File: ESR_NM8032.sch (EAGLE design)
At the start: 78 parts, among them J1 0

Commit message: .
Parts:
- C5: device rcl:CPOL-EUE2.5-5 -> rcl:CPOL-EUE2-5
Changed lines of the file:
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@@
 <grid distance="100" unitdist="mil" unit="mil" style="lines" multiple="1" display="yes" altdistance="0.01" altunitdist="inch" altunit="inch"/>
 <layers>
-<layer number="1" name="Top" color="4" fill="1" visible="no" active="no"/>
-<layer number="2" name="Route2" color="1" fill="3" visible="no" active="no"/>
-<layer number="3" name="Route3" color="4" fill="3" visible="no" active="no"/>
-<layer number="4" name="Route4" color="1" fill="4" visible="no" active="no"/>
-<layer number="5" name="Route5" color="4" fill="4" visible="no" active="no"/>
-<layer number="6" name="Route6" color="1" fill="8" visible="no" active="no"/>
-<layer number="7" name="Route7" color="4" fill="8" visible="no" active="no"/>
-<layer number="8" name="Route8" color="1" fill="2" visible="no" active="no"/>
-<layer number="9" name="Route9" color="4" fill="2" visible="no" active="no"/>
-<layer number="10" name="Route10" color="1" fill="7" visible="no" active="no"/>
-<layer number="11" name="Route11" color="4" fill="7" visible="no" active="no"/>
-<layer number="12" name="Route12" color="1" fill="5" visible="no" active="no"/>
-<layer number="13" name="Route13" color="4" fill="5" visible="no" active="no"/>
-<layer number="14" name="Route14" color="1" fill="6" visible="no" active="no"/>
-<layer number="15" name="Route15" color="4" fill="6" visible="no" active="no"/>
-<layer number="16" name="Bottom" color="1" fill="1" visible="no" active="no"/>
-<layer number="17" name="Pads" color="2" fill="1" visible="no" active="no"/>
-<layer number="18" name="Vias" color="2" fill="1" visible="no" active="no"/>
-<layer number="19" name="Unrouted" color="6" fill="1" visible="no" active="no"/>
-<layer number="20" name="Dimension" color="15" fill="1" visible="no" active="no"/>
-<layer number="21" name="tPlace" color="7" fill="1" visible="no" active="no"/>
-<layer number="22" name="bPlace" color="7" fill="1" visible="no" active="no"/>
-<layer number="23" name="tOrigins" color="15" fill="1" visible="no" active="no"/>
-<layer number="24" name="bOrigins" color="15" fill="1" visible="no" active="no"/>
-<layer number="25" name="tNames" color="7" fill="1" visible="no" active="no"/>
-<layer number="26" name="bNames" color="7" fill="1" visible="no" active="no"/>
-<layer number="27" name="tValues" color="7" fill="1" visible="no" active="no"/>
-<layer number="28" name="bValues" color="7" fill="1" visible="no" active="no"/>
+<layer number="1" name="Top" color="4" fill="1" visible="yes" active="no"/>
+<layer number="2" name="Route2" color="1" fill="3" visible="yes" active="no"/>
+<layer number="3" name="Route3" color="4" fill="3" visible="yes" active="no"/>
+<layer number="4" name="Route4" color="1" fill="4" visible="yes" active="no"/>
+<layer number="5" name="Route5" color="4" fill="4" visible="yes" active="no"/>
+<layer number="6" name="Route6" color="1" fill="8" visible="yes" active="no"/>
+<layer number="7" name="Route7" color="4" fill="8" visible="yes" active="no"/>
+<layer number="8" name="Route8" color="1" fill="2" visible="yes" active="no"/>
+<layer number="9" name="Route9" color="4" fill="2" visible="yes" active="no"/>
+<layer number="10" name="Route10" color="1" fill="7" visible="yes" active="no"/>
+<layer number="11" name="Route11" color="4" fill="7" visible="yes" active="no"/>
+<layer number="12" name="Route12" color="1" fill="5" visible="yes" active="no"/>
+<layer number="13" name="Route13" color="4" fill="5" visible="yes" active="no"/>
+<layer number="14" name="Route14" color="1" fill="6" visible="yes" active="no"/>
+<layer number="15" name="Route15" color="4" fill="6" visible="yes" active="no"/>
+<layer number="16" name="Bottom" color="1" fill="1" visible="yes" active="no"/>
+<layer number="17" name="Pads" color="2" fill="1" visible="yes" active="no"/>
+<layer number="18" name="Vias" color="2" fill="1" visible="yes" active="no"/>
+<layer number="19" name="Unrouted" color="6" fill="1" visible="yes" active="no"/>
+<layer number="20" name="Dimension" color="15" fill="1" visible="yes" active="no"/>
+<layer number="21" name="tPlace" color="7" fill="1" visible="yes" active="no"/>
+<layer number="22" name="bPlace" color="7" fill="1" visible="yes" active="no"/>
+<layer number="23" name="tOrigins" color="15" fill="1" visible="yes" active="no"/>
+<layer number="24" name="bOrigins" color="15" fill="1" visible="yes" active="no"/>
+<layer number="25" name="tNames" color="7" fill="1" visible="yes" active="no"/>
+<layer number="26" name="bNames" color="7" fill="1" visible="yes" active="no"/>
+<layer number="27" name="tValues" color="7" fill="1" visible="yes" active="no"/>
+<layer number="28" name="bValues" color="7" fill="1" visible="yes" active="no"/>
 <layer number="29" name="tStop" color="7" fill="3" visible="no" active="no"/>
 <layer number="30" name="bStop" color="7" fill="6" visible="no" active="no"/>
@@
 <layer number="35" name="tGlue" color="7" fill="4" visible="no" active="no"/>
 <layer number="36" name="bGlue" color="7" fill="5" visible="no" active="no"/>
-<layer number="37" name="tTest" color="7" fill="1" visible="no" active="no"/>
-<layer number="38" name="bTest" color="7" fill="1" visible="no" active="no"/>
+<layer number="37" name="tTest" color="7" fill="1" visible="yes" active="no"/>
+<layer number="38" name="bTest" color="7" fill="1" visible="yes" active="no"/>
 <layer number="39" name="tKeepout" color="4" fill="11" visible="no" active="no"/>
 <layer number="40" name="bKeepout" color="1" fill="11" visible="no" active="no"/>
@@
 <layer number="44" name="Drills" color="7" fill="1" visible="no" active="no"/>
 <layer number="45" name="Holes" color="7" fill="1" visible="no" active="no"/>
-<layer number="46" name="Milling" color="3" fill="1" visible="no" active="no"/>
-<layer number="47" name="Measures" color="7" fill="1" visible="no" active="no"/>
-<layer number="48" name="Document" color="7" fill="1" visible="no" active="no"/>
-<layer number="49" name="Reference" color="7" fill="1" visible="no" active="no"/>
-<layer number="50" name="dxf" color="7" fill="1" visible="no" active="no"/>
-<layer number="51" name="tDocu" color="7" fill="1" visible="no" active="no"/>
-<layer number="52" name="bDocu" color="7" fill="1" visible="no" active="no"/>
-<layer number="53" name="tGND_GNDA" color="7" fill="9" visible="no" active="no"/>
-<layer number="54" name="bGND_GNDA" color="1" fill="9" visible="no" active="no"/>
-<layer number="56" name="wert" color="7" fill="1" visible="no" active="no"/>
-<layer number="57" name="tCAD" color="7" fill="1" visible="no" active="no"/>
+<layer number="46" name="Milling" color="3" fill="1" visible="yes" active="no"/>
+<layer number="47" name="Measures" color="7" fill="1" visible="yes" active="no"/>
+<layer number="48" name="Document" color="7" fill="1" visible="yes" active="no"/>
+<layer number="49" name="Reference" color="7" fill="1" visible="yes" active="no"/>
+<layer number="50" name="dxf" color="7" fill="1" visible="yes" active="no"/>
+<layer number="51" name="tDocu" color="7" fill="1" visible="yes" active="no"/>
+<layer number="52" name="bDocu" color="7" fill="1" visible="yes" active="no"/>
+<layer number="53" name="tGND_GNDA" color="7" fill="9" visible="yes" active="no"/>
+<layer number="54" name="bGND_GNDA" color="1" fill="9" visible="yes" active="no"/>
+<layer number="56" name="wert" color="7" fill="1" visible="yes" active="no"/>
+<layer number="57" name="tCAD" color="7" fill="1" visible="yes" active="no"/>
 <layer number="90" name="Modules" color="5" fill="1" visible="yes" active="yes"/>
 <layer number="91" name="Nets" color="2" fill="1" visible="yes" active="yes"/>
@@
 <part name="R8" library="rcl" deviceset="R-EU_" device="R0805" value="10k"/>
 <part name="GND5" library="supply1" deviceset="GND" device=""/>
-<part name="C5" library="rcl" deviceset="CPOL-EU" device="E2.5-5" value="10m"/>
+<part name="C5" library="rcl" deviceset="CPOL-EU" device="E2-5" value="10m"/>
 <part name="R7" library="rcl" deviceset="R-EU_" device="R0805" value="10k"/>
 <part name="C6" library="rcl" deviceset="C-EU" device="075-032X103" value="220n"/>

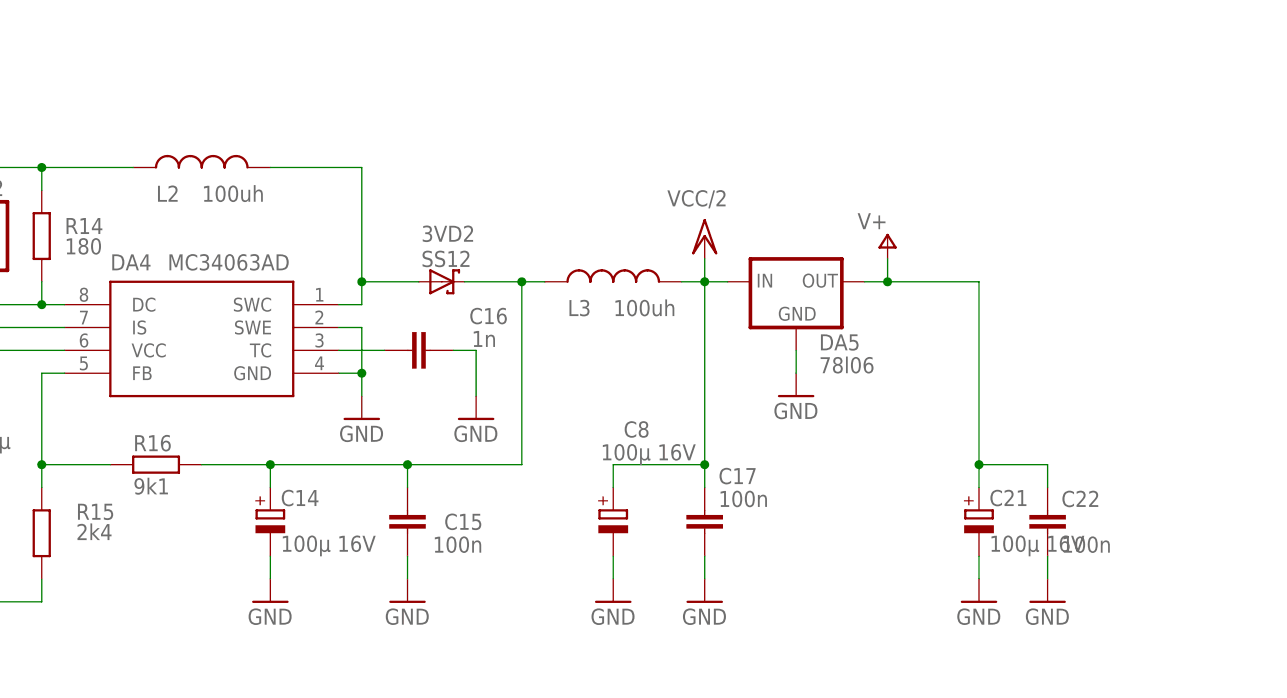
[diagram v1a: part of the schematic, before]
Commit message: .
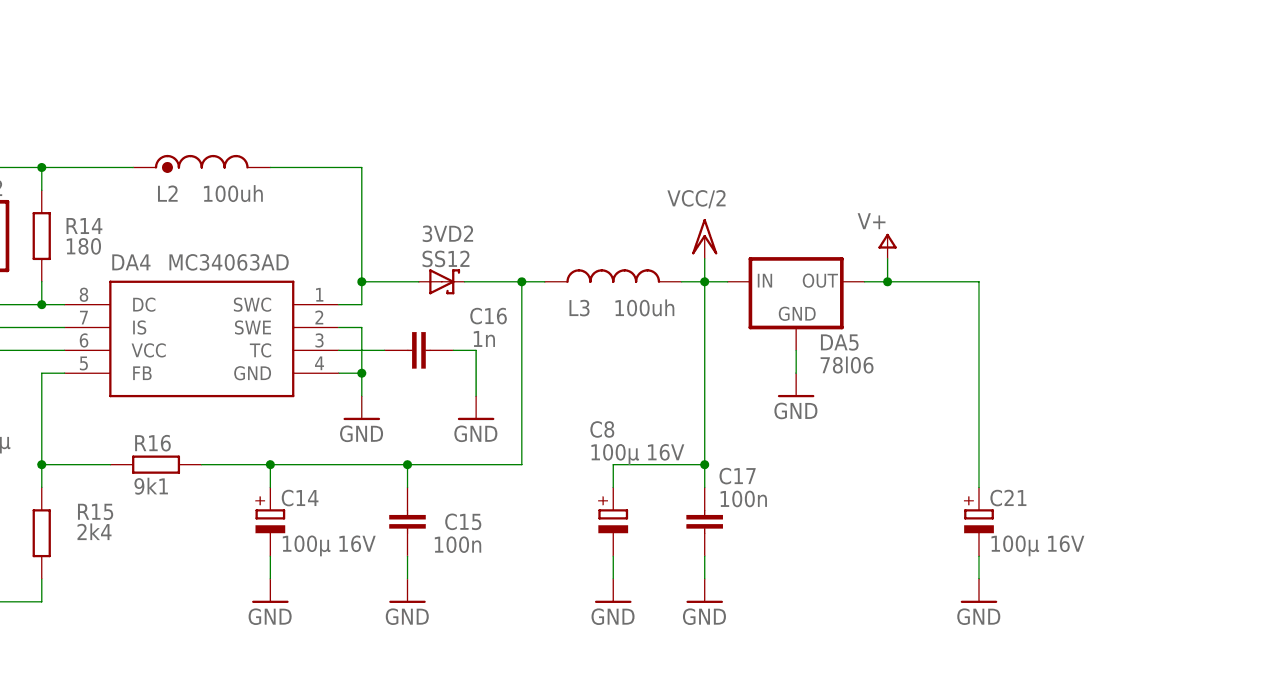
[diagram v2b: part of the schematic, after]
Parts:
- removed C22: 100n, rcl:C-EUC0805
- X1, X2: device pinhead:PINHD-1X2 -> Разъёмы штырьковые 2.54мм:PINHD-1X2/2
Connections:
- net GND: no longer C22.2
- net V+: no longer C22.1
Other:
- note added: "C22 100n"
